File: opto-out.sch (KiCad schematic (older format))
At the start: 4 parts, among them Q8 BC817, U4 4N25

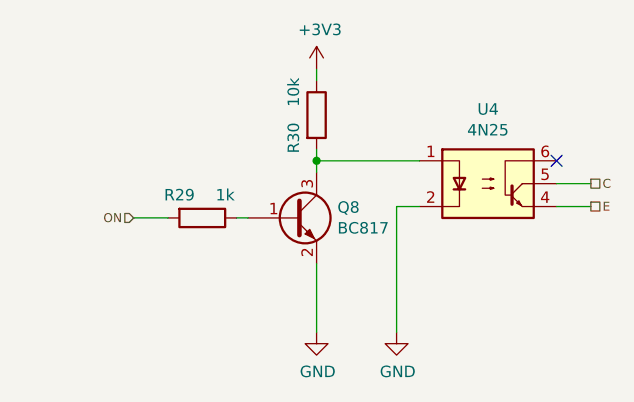
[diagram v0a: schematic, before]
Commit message: Several changes
Usando stock de http://tienda.ityt.com.ar/
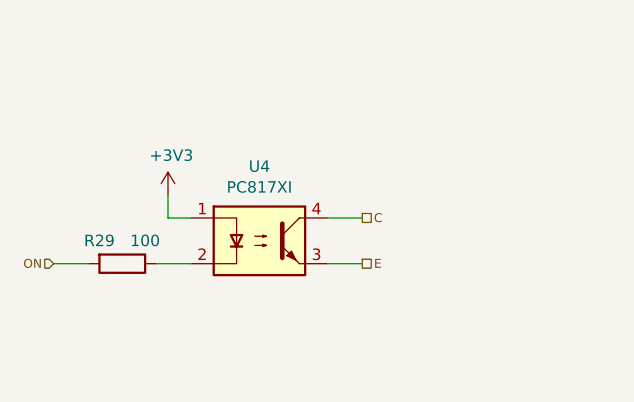
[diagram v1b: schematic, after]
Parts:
- removed Q8: BC817, Package_TO_SOT_SMD:SOT-23, symbol Transistor_BJT:BC817
- removed R30: 10k, Resistor_SMD:R_1206_3216Metric, symbol Device:R
- removed U4: 4N25, Package_DIP:DIP-6_W7.62mm, symbol Isolator:4N25
- added U4: PC817XI, Package_DIP:SMDIP-4_W9.53mm, symbol Isolator:PC817
- R29: value 1k -> 100; manf# RC1206FR-071KL -> RC1206FR-07100RL
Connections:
- net +3V3: now also U4.1
- net C: now also U4.4
- net E: now also U4.3
- net at R29.1: now also U4.2
- no-connect marks 1 -> 0
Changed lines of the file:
@@
 $Descr A4 11693 8268
 encoding utf-8
-Sheet 16 19
+Sheet 15 18
 Title "Opto-coupled Output"
 Date "2021-06-10"
@@
 $EndDescr
 $Comp
-L Isolator:4N25 U?
-U 1 1 6149516B
-P 6450 3700
-AR Path="/6149516B" Ref="U?"  Part="1"
-AR Path="/61400494/61448E8E/6149516B" Ref="U4"  Part="1"
-AR Path="/61400494/614555D4/6149516B" Ref="U?"  Part="1"
-F 0 "U4" H 6450 4025 50  0000 C CNN
-F 1 "4N25" H 6450 3934 50  0000 C CNN
-F 2 "Package_DIP:DIP-6_W7.62mm" H 6250 3500 50  0001 L CIN
-F 3 "https://optoelectronics.liteon.com/upload/download/DS-70-99-0010/4N2X%20series%20Datasheet%201115.pdf" H 6450 3700 50  0001 L CNN
-F 4 "4N25" H 6450 3700 50  0001 C CNN "manf#"
-	1    6450 3700
-	1    0    0    -1
+L Device:R R?
+U 1 1 60DE53EE
+P 4850 4050
+AR Path="/60DE53EE" Ref="R?"  Part="1"
+AR Path="/61400494/61448E8E/60DE53EE" Ref="R?"  Part="1"
+AR Path="/61400494/614555D4/60DE53EE" Ref="R?"  Part="1"
+AR Path="/60DA21CE/60DE53EE" Ref="R29"  Part="1"
+F 0 "R29" V 4750 3950 50  0000 C CNN
+F 1 "100" V 4750 4150 50  0000 C CNN
+F 2 "Resistor_SMD:R_1206_3216Metric" V 4780 4050 50  0001 C CNN
+F 3 "https://www.yageo.com/upload/media/product/productsearch/datasheet/rchip/PYu-RC_Group_51_RoHS_L_11.pdf" H 4850 4050 50  0001 C CNN
+F 4 "RC1206FR-07100RL" H 4850 4050 50  0001 C CNN "manf#"
+	1    4850 4050
+	0    1    1    0
 $EndComp
+Text HLabel 4550 4050 0    39   Input ~ 0
+ON
+Text HLabel 5900 3850 2    39   UnSpc ~ 0
+C
+Text HLabel 5900 4050 2    39   UnSpc ~ 0
+E
+Wire Wire Line
+	5900 3850 5750 3850
+Wire Wire Line
+	5750 4050 5900 4050
 $Comp
-L power:GND #PWR?
-U 1 1 6144C51B
-P 5700 4350
-AR Path="/6144C51B" Ref="#PWR?"  Part="1"
-AR Path="/61400494/61448E8E/6144C51B" Ref="#PWR0148"  Part="1"
-AR Path="/61400494/614555D4/6144C51B" Ref="#PWR?"  Part="1"
-F 0 "#PWR0148" H 5700 4100 50  0001 C CNN
-F 1 "GND" H 5705 4177 50  0000 C CNN
-F 2 "" H 5700 4350 50  0001 C CNN
-F 3 "" H 5700 4350 50  0001 C CNN
-	1    5700 4350
+L power:+3V3 #PWR?
+U 1 1 60DE62E6
+P 5050 3750
+AR Path="/60DE62E6" Ref="#PWR?"  Part="1"
+AR Path="/61400494/61448E8E/60DE62E6" Ref="#PWR?"  Part="1"
+AR Path="/61400494/614555D4/60DE62E6" Ref="#PWR?"  Part="1"
+AR Path="/60DA21CE/60DE62E6" Ref="#PWR0147"  Part="1"
+F 0 "#PWR0147" H 5050 3600 50  0001 C CNN
+F 1 "+3V3" H 5065 3923 50  0000 C CNN
+F 2 "" H 5050 3750 50  0001 C CNN
+F 3 "" H 5050 3750 50  0001 C CNN
+	1    5050 3750
 	1    0    0    -1
 $EndComp
 Wire Wire Line
-	5400 3850 5350 3850
+	5050 3750 5050 3850
+Wire Wire Line
+	5050 3850 5150 3850
+Wire Wire Line
+	5150 4050 5000 4050
+Wire Wire Line
+	4700 4050 4550 4050
 $Comp
-L Device:R R?
-U 1 1 6144C525
-P 5200 3850
-AR Path="/6144C525" Ref="R?"  Part="1"
-AR Path="/61400494/61448E8E/6144C525" Ref="R29"  Part="1"
-AR Path="/61400494/614555D4/6144C525" Ref="R?"  Part="1"
-F 0 "R29" V 5100 3750 50  0000 C CNN
-F 1 "1k" V 5100 3950 50  0000 C CNN
-F 2 "Resistor_SMD:R_1206_3216Metric" V 5130 3850 50  0001 C CNN
-F 3 "https://www.yageo.com/upload/media/product/productsearch/datasheet/rchip/PYu-RC_Group_51_RoHS_L_11.pdf" H 5200 3850 50  0001 C CNN
-F 4 "RC1206FR-071KL" H 5200 3850 50  0001 C CNN "manf#"
-	1    5200 3850
-	0    1    1    0
-$EndComp
-$Comp
-L Transistor_BJT:BC817 Q?
-U 1 1 6144C52B
-P 5600 3850
-AR Path="/6144C52B" Ref="Q?"  Part="1"
-AR Path="/61400494/61448E8E/6144C52B" Ref="Q8"  Part="1"
-AR Path="/61400494/614555D4/6144C52B" Ref="Q?"  Part="1"
-F 0 "Q8" H 5791 3896 50  0000 L CNN
-F 1 "BC817" H 5791 3805 50  0000 L CNN
-F 2 "Package_TO_SOT_SMD:SOT-23" H 5800 3775 50  0001 L CIN
-F 3 "https://www.onsemi.com/pub/Collateral/BC817-16LT1-D.PDF" H 5600 3850 50  0001 L CNN
-F 4 "SBC817-40LT1G" H 5600 3850 50  0001 C CNN "manf#"
-	1    5600 3850
+L Isolator:PC817 U4
+U 1 1 60DC3AB9
+P 5450 3950
+F 0 "U4" H 5450 4275 50  0000 C CNN
+F 1 "PC817XI" H 5450 4184 50  0000 C CNN
+F 2 "Package_DIP:SMDIP-4_W9.53mm" H 5250 3750 50  0001 L CIN
+F 3 "https://www.farnell.com/datasheets/73758.pdf" H 5450 3950 50  0001 L CNN
+F 4 "PC817XI" H 5450 3950 50  0001 C CNN "manf#"
+	1    5450 3950
 	1    0    0    -1
 $EndComp
-Wire Wire Line
-	5700 3650 5700 3600
-$Comp
-L Device:R R?
-U 1 1 6144C532
-P 5700 3400
-AR Path="/6144C532" Ref="R?"  Part="1"
-AR Path="/61400494/61448E8E/6144C532" Ref="R30"  Part="1"
-AR Path="/61400494/614555D4/6144C532" Ref="R?"  Part="1"
-F 0 "R30" V 5600 3300 50  0000 C CNN
-F 1 "10k" V 5600 3500 50  0000 C CNN
-F 2 "Resistor_SMD:R_1206_3216Metric" V 5630 3400 50  0001 C CNN
-F 3 "https://www.yageo.com/upload/media/product/productsearch/datasheet/rchip/PYu-RC_Group_51_RoHS_L_11.pdf" H 5700 3400 50  0001 C CNN
-F 4 "RC1206FR-0710KL" H 5700 3400 50  0001 C CNN "manf#"
-	1    5700 3400
-	1    0    0    -1
-$EndComp
-$Comp
-L power:+3V3 #PWR?
-U 1 1 6149516C
-P 5700 3200
-AR Path="/6149516C" Ref="#PWR?"  Part="1"
-AR Path="/61400494/61448E8E/6149516C" Ref="#PWR0149"  Part="1"
-AR Path="/61400494/614555D4/6149516C" Ref="#PWR?"  Part="1"
-F 0 "#PWR0149" H 5700 3050 50  0001 C CNN
-F 1 "+3V3" H 5715 3373 50  0000 C CNN
-F 2 "" H 5700 3200 50  0001 C CNN
-F 3 "" H 5700 3200 50  0001 C CNN
-	1    5700 3200
-	1    0    0    -1
-$EndComp
-Wire Wire Line
-	5700 3250 5700 3200
-Wire Wire Line
-	6150 3600 5700 3600
-Connection ~ 5700 3600
-Wire Wire Line
-	5700 3600 5700 3550
-Wire Wire Line
-	6050 3800 6150 3800
-NoConn ~ 6750 3600
-Wire Wire Line
-	5700 4050 5700 4350
-$Comp
-L power:GND #PWR?
-U 1 1 6144CC46
-P 6050 4350
-AR Path="/6144CC46" Ref="#PWR?"  Part="1"
-AR Path="/61400494/61448E8E/6144CC46" Ref="#PWR0150"  Part="1"
-AR Path="/61400494/614555D4/6144CC46" Ref="#PWR?"  Part="1"
-F 0 "#PWR0150" H 6050 4100 50  0001 C CNN
-F 1 "GND" H 6055 4177 50  0000 C CNN
-F 2 "" H 6050 4350 50  0001 C CNN
-F 3 "" H 6050 4350 50  0001 C CNN
-	1    6050 4350
-	1    0    0    -1
-$EndComp
-Wire Wire Line
-	6050 4350 6050 3800
-Text HLabel 4900 3850 0    39   Input ~ 0
-ON
-Wire Wire Line
-	4900 3850 5050 3850
-Text HLabel 6900 3700 2    39   UnSpc ~ 0
-C
-Text HLabel 6900 3800 2    39   UnSpc ~ 0
-E
-Wire Wire Line
-	6900 3700 6750 3700
-Wire Wire Line
-	6750 3800 6900 3800
 $EndSCHEMATC
